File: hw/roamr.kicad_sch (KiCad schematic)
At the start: 18 parts, among them U1 TPS56A37RPAR

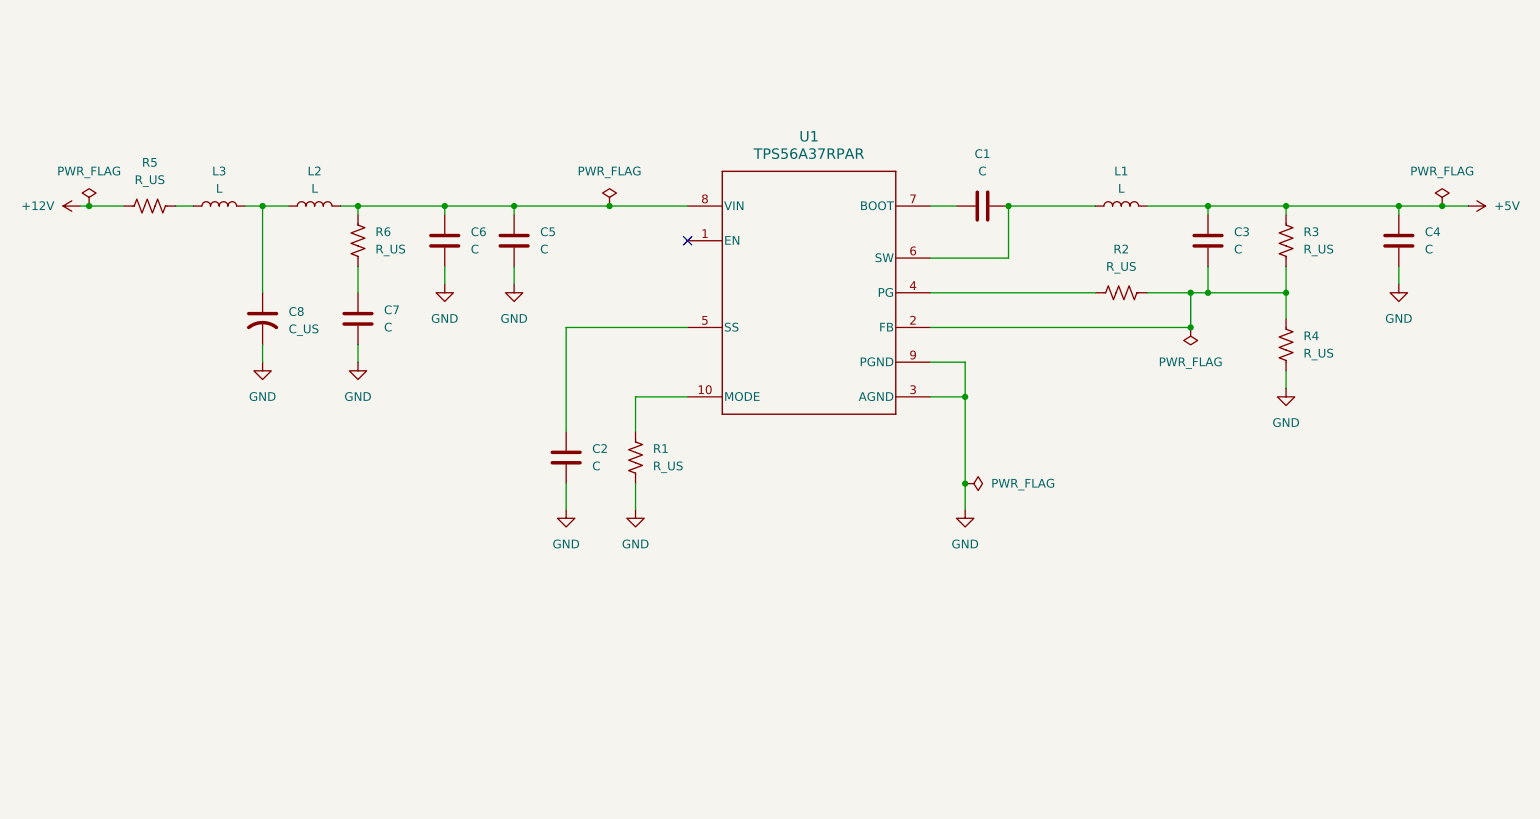
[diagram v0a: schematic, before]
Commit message: olivia's edits
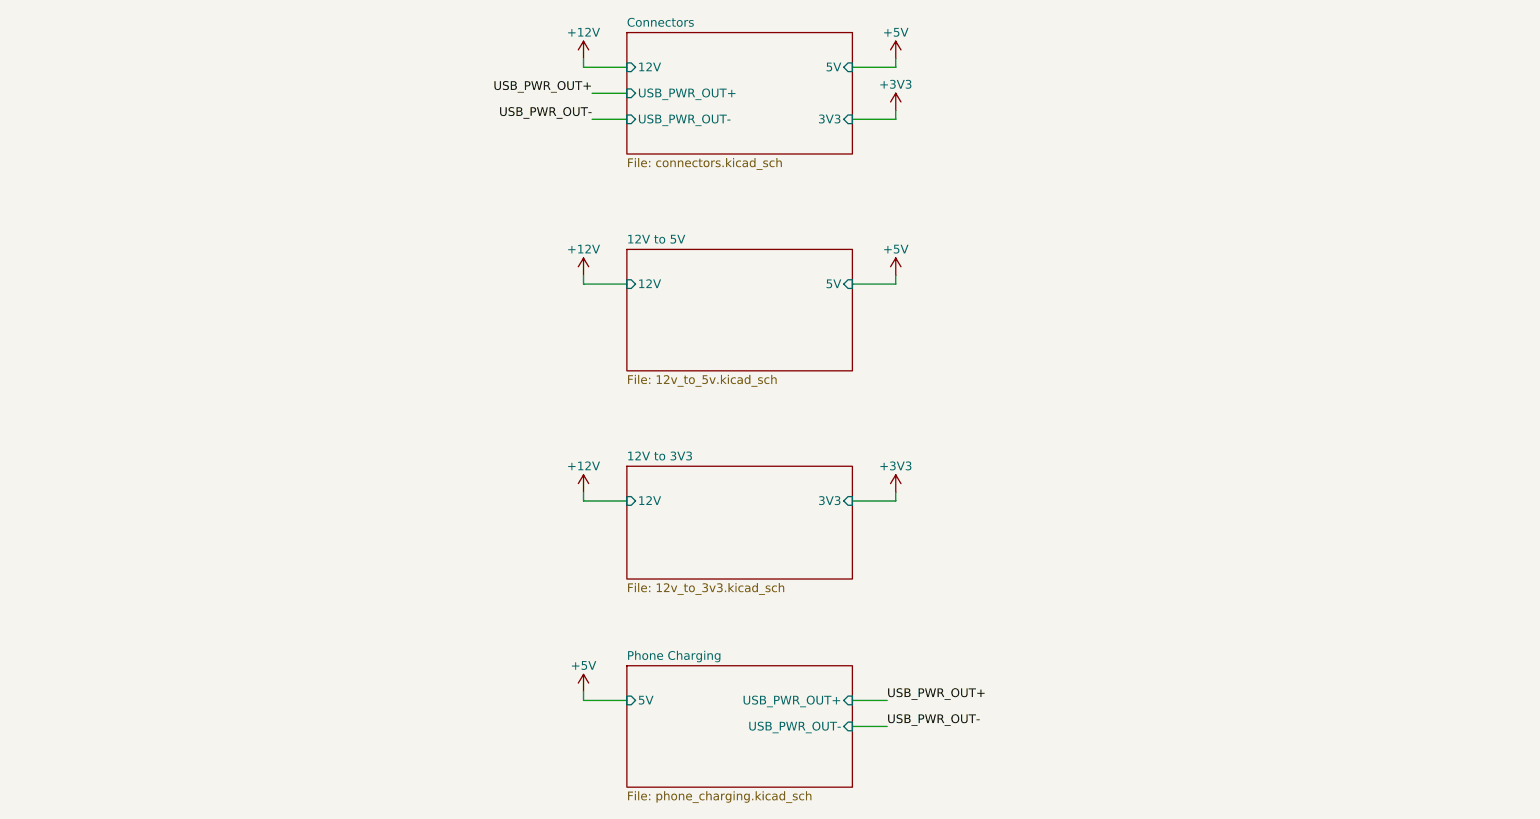
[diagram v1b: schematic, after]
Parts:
- removed C1, C2, C3, C4, C5, C6, C7: C, symbol Device:C
- removed C8: C_US, symbol Device:C_US
- removed L1, L2, L3: L, symbol Device:L
- removed R1, R2, R3, R4, R5, R6: R_US, symbol Device:R_US
- removed U1: TPS56A37RPAR, TPS56A37RPAR:RPA0010A-MFG, symbol TPS56A37RPAR:TPS56A37RPAR
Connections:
- no-connect marks 1 -> 0
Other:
- added sheet 12V to 3V3 (12v_to_3v3.kicad_sch)
- added sheet 12V to 5V (12v_to_5v.kicad_sch)
- added sheet Connectors (connectors.kicad_sch)
- added sheet Phone Charging (phone_charging.kicad_sch)
